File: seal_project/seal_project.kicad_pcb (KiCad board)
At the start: 2 copper layers, 3 parts

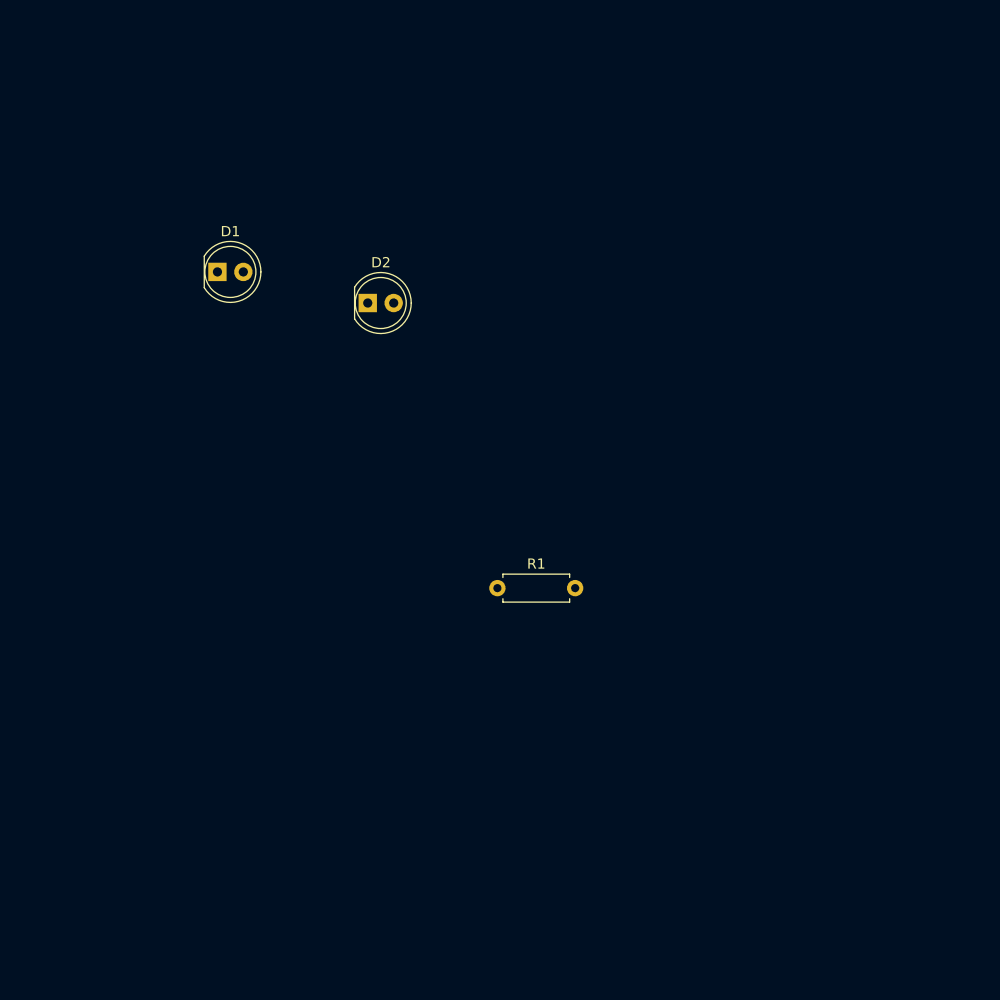
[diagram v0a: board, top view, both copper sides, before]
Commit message: updated files
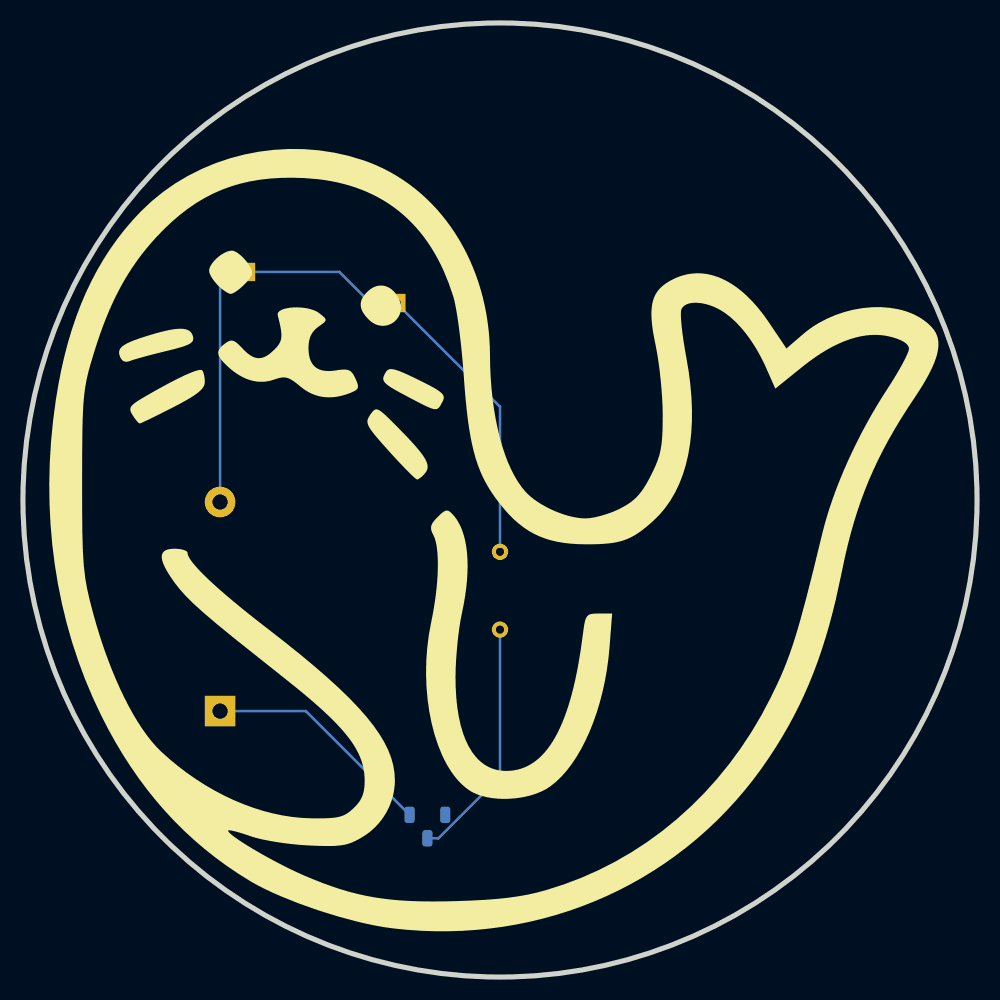
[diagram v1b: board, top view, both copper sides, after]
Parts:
- added BT1: Battery_Cell, Battery:BatteryHolder_Keystone_106_1x20mm, B.Cu at (130.0, 116.2)
- added SW1: SW_SPDT, Button_Switch_SMD:Nidec_Copal_CAS-120A, B.Cu at (150.4, 127.5)
- D1, D2, R1: moved to B.Cu
- moved R1 4.07 mm to (157.5, 108.2), turned to 90 degrees
- moved D1 2.80 mm to (132.6, 73.2), turned to 180 degrees
- moved D2 2.80 mm to (147.3, 76.2), turned to 180 degrees
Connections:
- D1 pad 2: Net-(D1-A) -> Net-(BT1--)
- D2 pad 1: Net-(D1-A) -> Net-(D2-K)
- D2 pad 2: Net-(D2-A) -> Net-(D1-K)
- R1 pad 1: Net-(D2-A) -> Net-(SW1-B)
- R1 pad 2: Net-(BT1--) -> Net-(D2-K)
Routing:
- net Net-(D2-K): track 0.00 -> 28.6 mm
- net Net-(SW1-B): track 0.00 -> 24.0 mm
- net Net-(BT1-+): track 0.00 -> 22.8 mm
- net Net-(BT1--): track 0.00 -> 22.5 mm
- net Net-(D1-K): track 0.00 -> 13.5 mm
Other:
- board outline added: 93.5 x 93.5 mm
- board text added: "To: Ezzat From: Cal"
